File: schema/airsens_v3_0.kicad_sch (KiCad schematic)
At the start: 36 parts, among them J1 ALIM, J3 USB TO UART, J4 PAIR, J5 LED, U1 MAX604, U2 ESP32-WROOM-32, U3 PAIR-IO12, j2 BME280

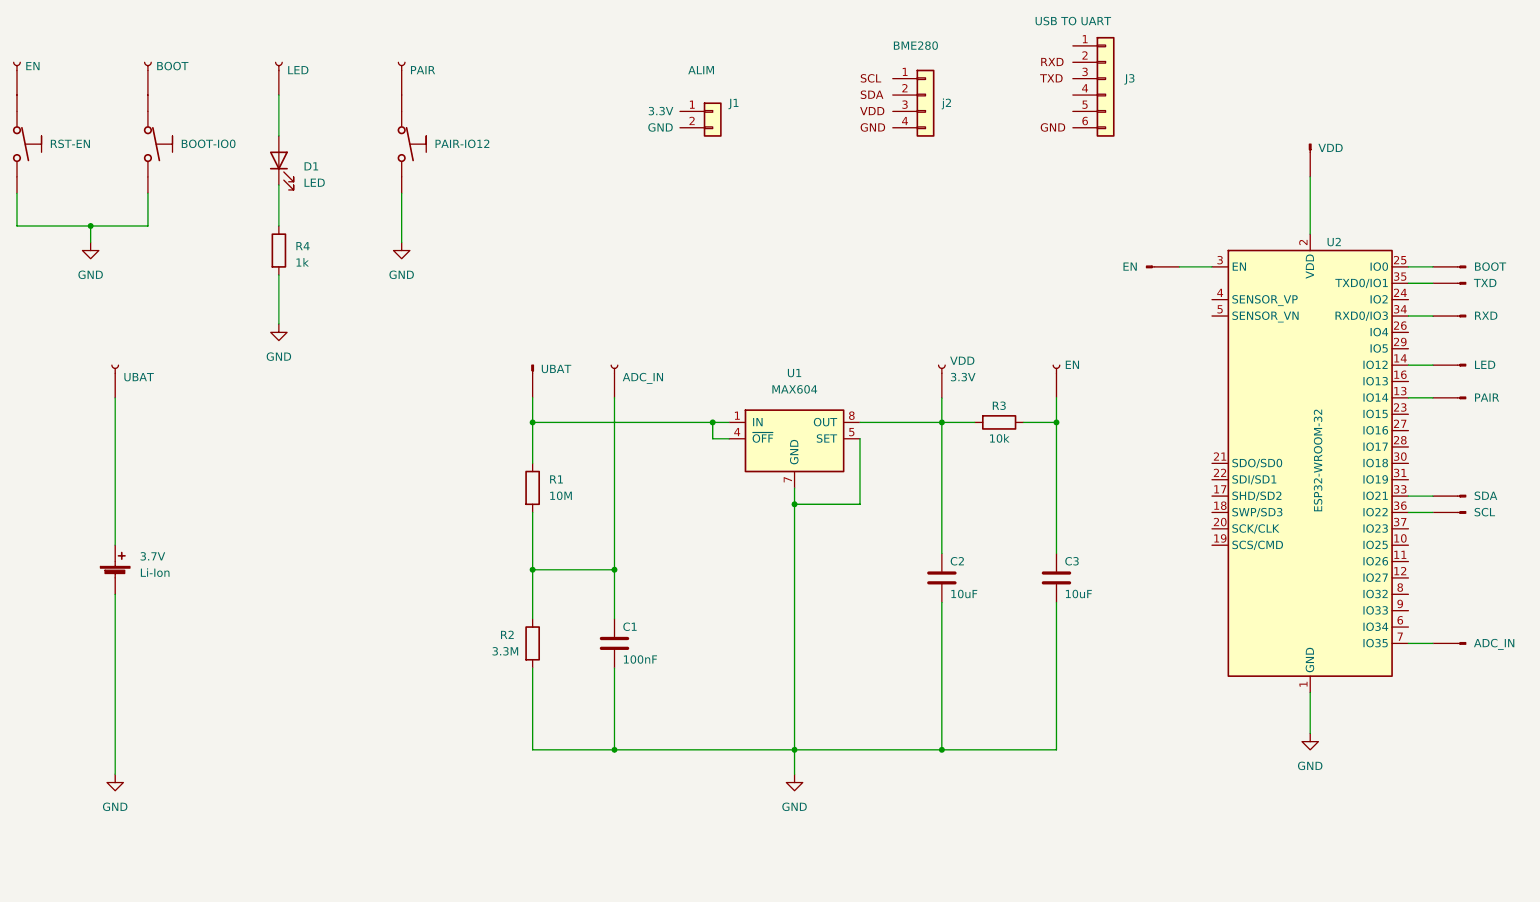
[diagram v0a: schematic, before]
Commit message: Ready for the hardware
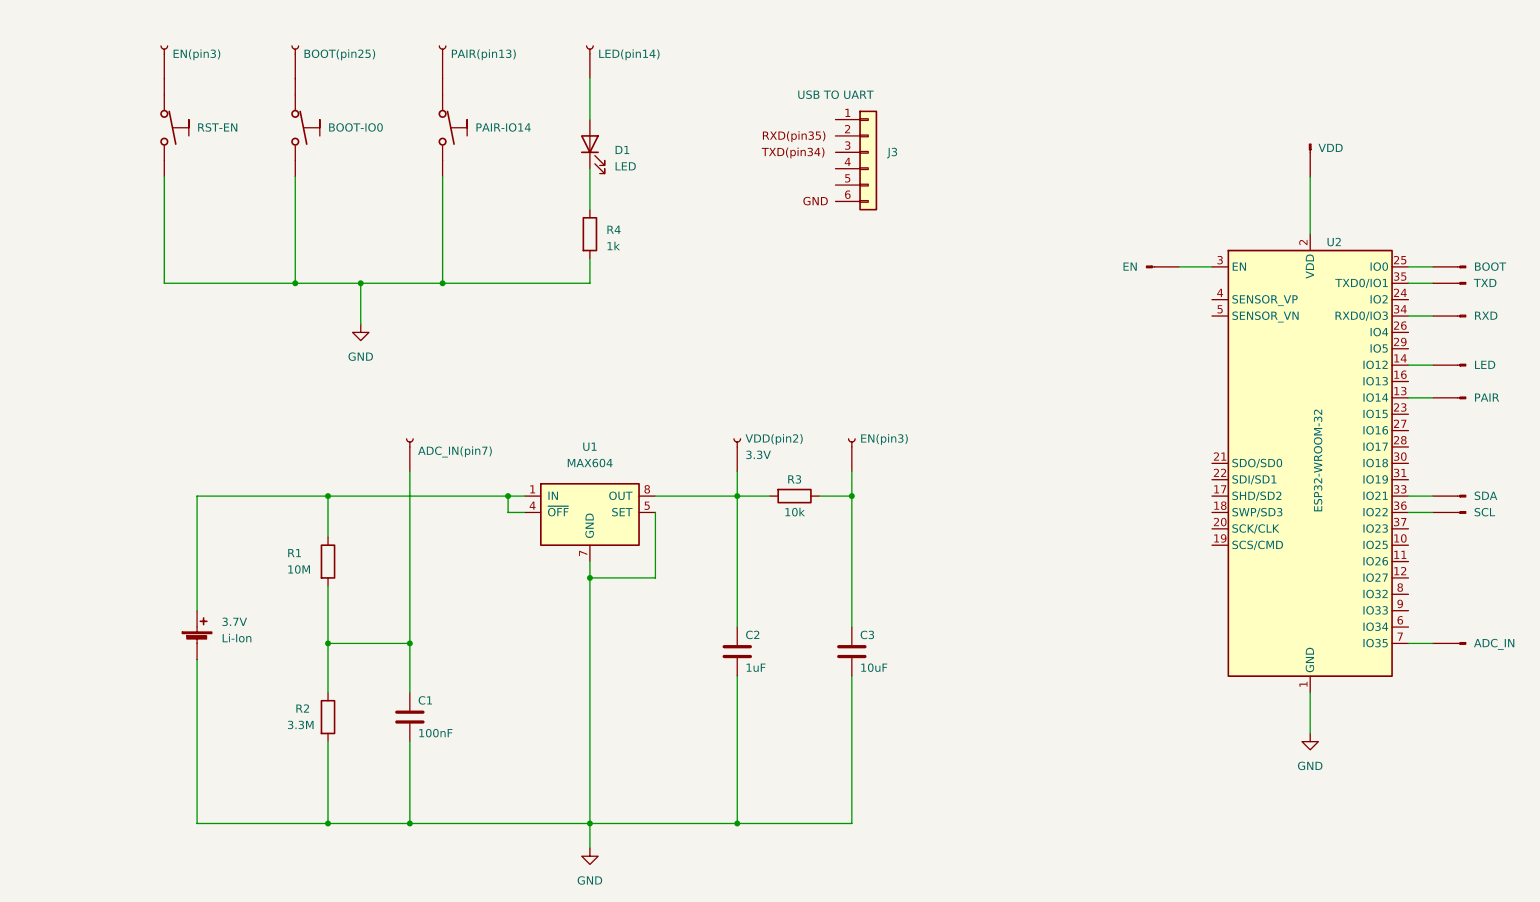
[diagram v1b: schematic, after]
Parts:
- removed J1: ALIM, symbol Connector_Generic:Conn_01x02
- removed J?: UBAT, symbol Connector:Conn_01x01_Male
- removed J?: UBAT, symbol Connector:Conn_01x01_Female
- removed LED: EN, symbol Connector:Conn_01x01_Female
- removed j2: BME280, symbol Connector_Generic:Conn_01x04
- added LED(pin14): EN, symbol Connector:Conn_01x01_Female
- C2: value 10uF -> 1uF
- J?: value ADC_IN -> ADC_IN(pin7)
- U3: value PAIR-IO12 -> PAIR-IO14
- renumbered BOOT to BOOT(pin25), EN to EN(pin3), PAIR to PAIR(pin13), VDD to VDD(pin2)
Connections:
- net at 3.7V.1 (+): now also R1.1, U1.1 (IN), U1.4 (~{OFF})
- net at D1.2 (A): now also LED(pin14).1 (Pin_1)
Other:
- moved on the sheet: 3.7V, BOOT(pin25), C1, C2, C3, EN(pin3), J3, PAIR(pin13), R1, R2, R3, U1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
